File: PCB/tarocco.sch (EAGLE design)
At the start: 42 parts, among them IC1 CY8C4545PVI, Q1 NEXFET_SINGLECSD18537NQ5A, Q2 NEXFET_SINGLECSD18537NQ5A, Q3 NEXFET_SINGLECSD18537NQ5A, Q4 NEXFET_SINGLECSD18537NQ5A

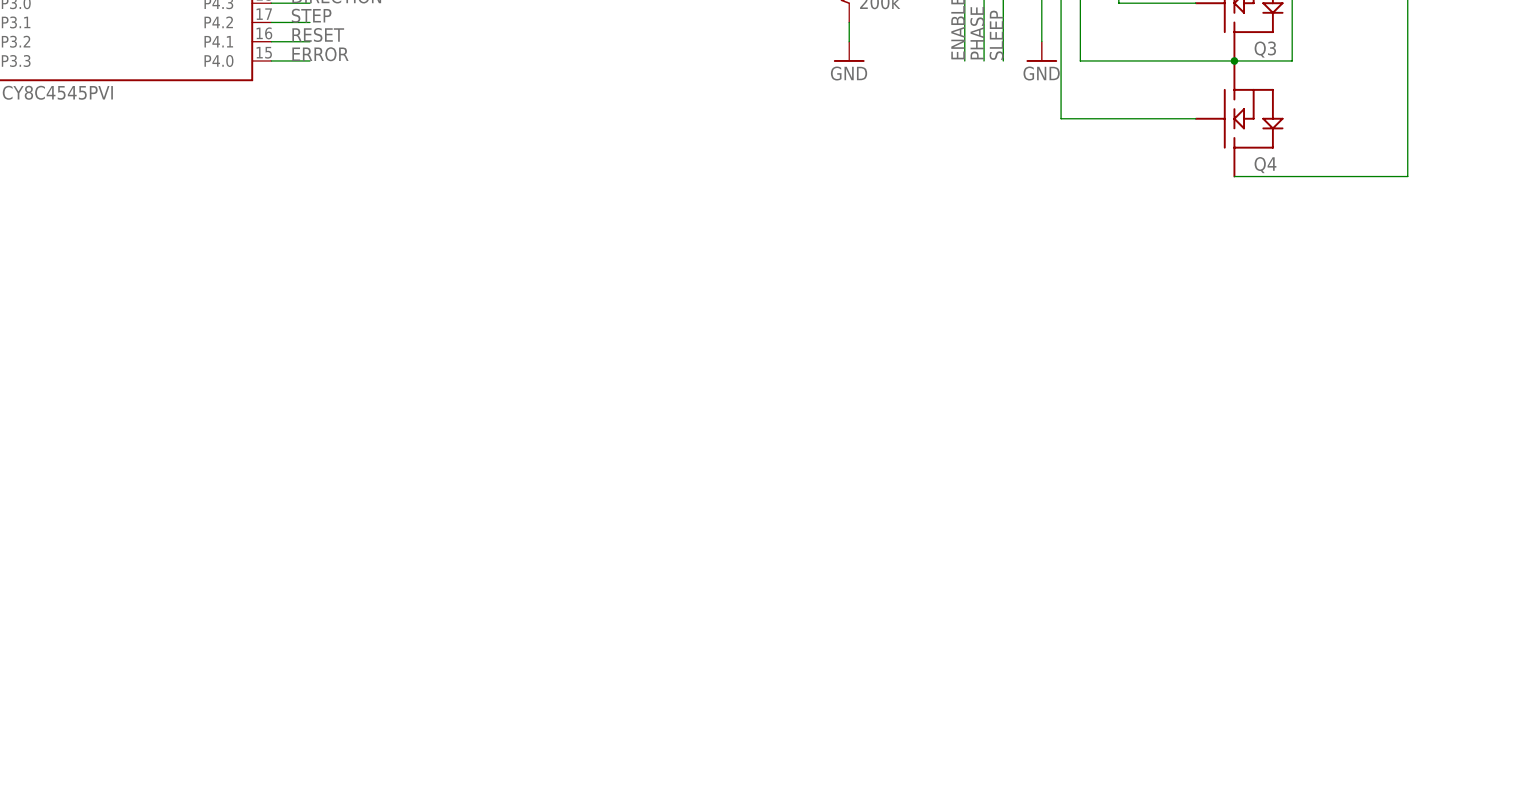
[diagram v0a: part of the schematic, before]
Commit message: Initial Commit of Schematic
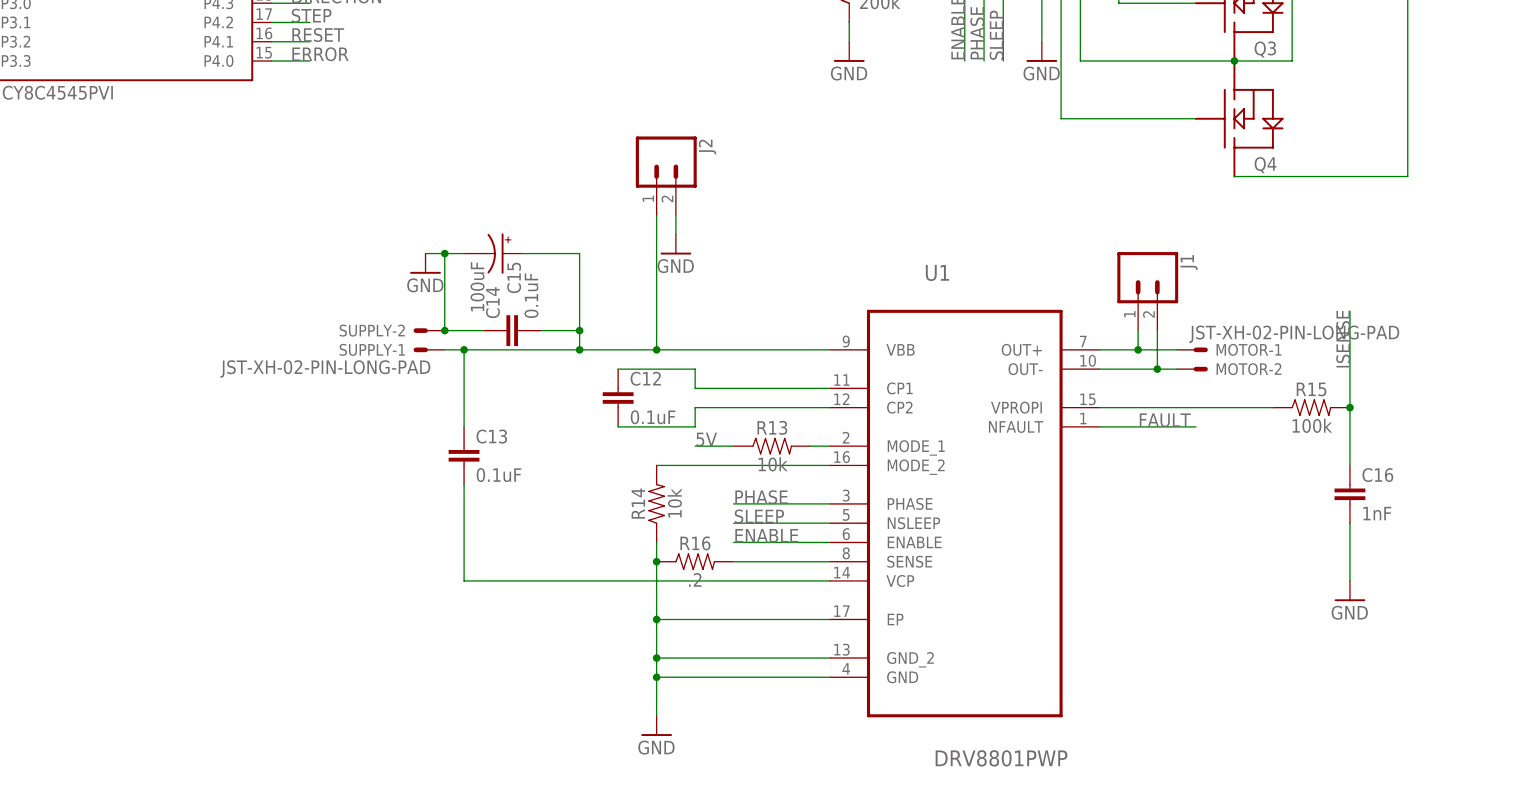
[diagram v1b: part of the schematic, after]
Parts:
- added C12: 0.1uF, SparkFun-Capacitors:0.1UF-0603-100V-10%
- added C13, C14: 0.1uF, SparkFun-Capacitors:0.1UF-0603-25V-(+80/-20%)
- added C15: 100uF, SparkFun-Capacitors:100UF-POLAR-RADIAL-2.5MM-25V-20%
- added C16: 1nF, SparkFun-Capacitors:1.0NF/1000PF-0603-50V-10%
- added J1, J2: (no value), SparkFun-Connectors:CONN_02PTH3
- added MOTOR, SUPPLY: JST-XH-02-PIN-LONG-PAD, JST XH Connectors v1-0:JST-XH-02-PIN-LONG-PAD
- added R13, R14: 10k, SparkFun-Resistors:10KOHM-0603-1/10W-1%
- added R15: 100k, SparkFun-Resistors:100KOHM-0603-1/10W-1%
- added R16: .2, SparkFun-Resistors:510OHM-2010-1/2W-5%
- added U1: DRV8801PWP, DRV8801PWP:DRV8801PWP
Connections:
- new net N$26: C13.1, C14.2, C15.+, J2.1, SUPPLY-1.S, U1.VBB
- new net N$27: R15.1, U1.VPROPI
- new net N$28: C12.1, U1.CP1
- new net N$30: C12.2, U1.CP2
- new net N$31: C13.2, U1.VCP
- new net N$32: R14.2, U1.MODE_2
- new net N$36: R16.2, U1.SENSE
- new net N$37: J1.1, MOTOR-1.S, U1.OUT+
- new net N$38: J1.2, MOTOR-2.S, U1.OUT-
- new net N$9: R13.2, U1.MODE_1
- net 5V: now also R13.1
- net ENABLE: now also U1.ENABLE
- net FAULT: now also U1.NFAULT
- net GND: now also C14.1, C15.-, C16.2, J2.2, R14.1, R16.1, SUPPLY-2.S, U1.EP, U1.GND, U1.GND_2
- net ISENSE: now also C16.1, R15.2
- net PHASE: now also U1.PHASE
- net SLEEP: now also U1.NSLEEP

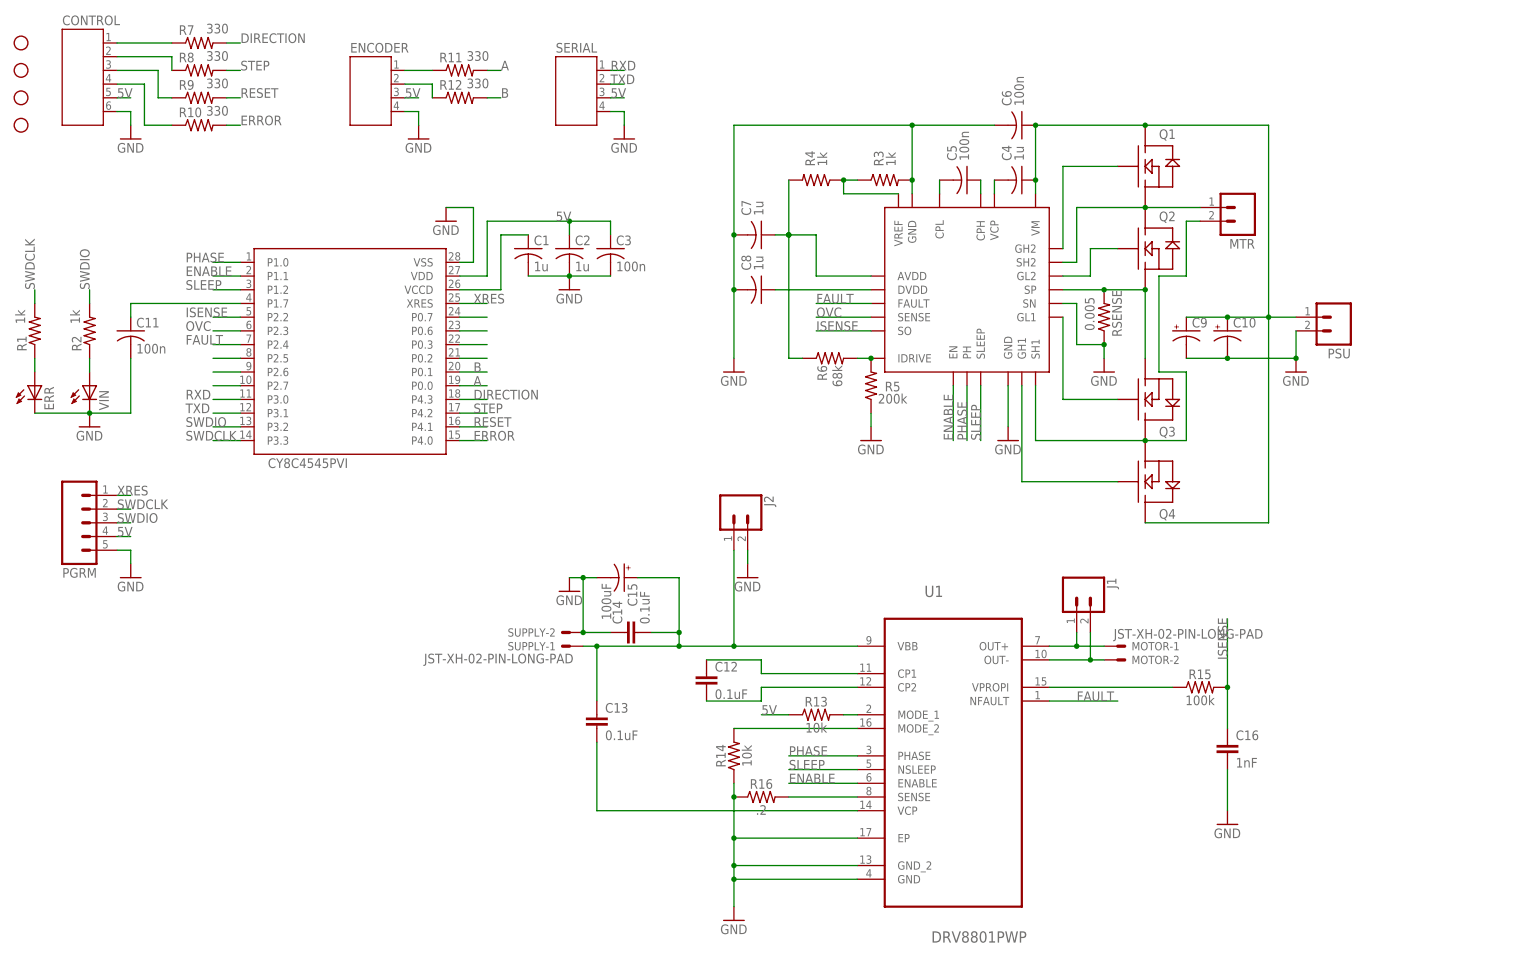
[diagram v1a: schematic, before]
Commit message: Starting BRD from scratch
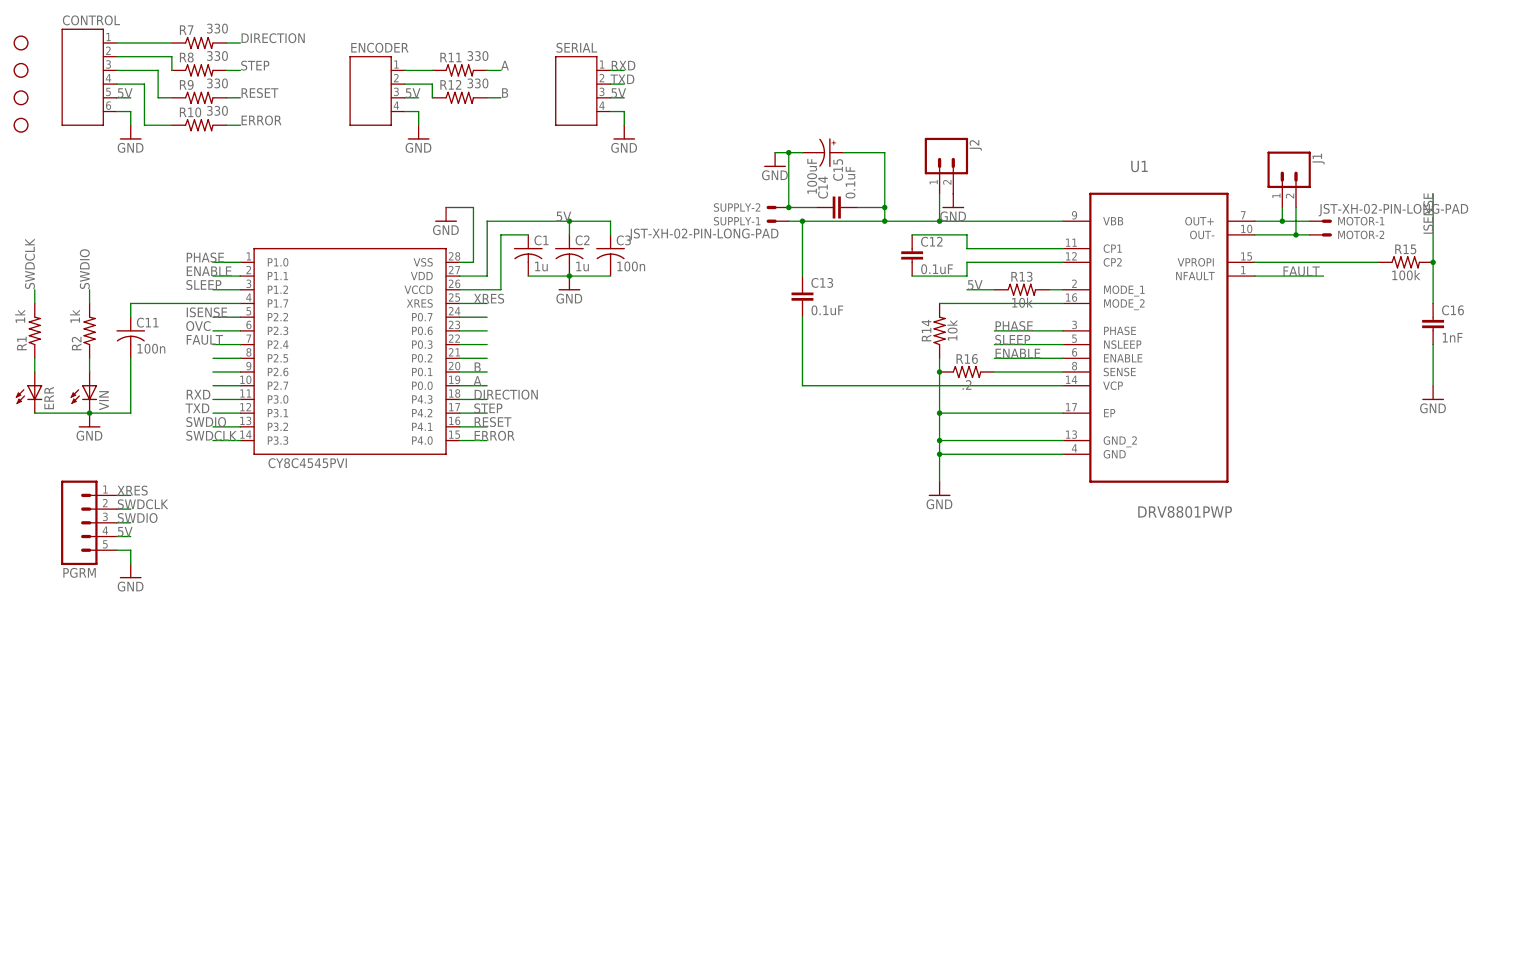
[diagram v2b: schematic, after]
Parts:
- removed 8701: DRV8701, drv8x:DRV8701
- removed C10, C9: (no value), adafruit:CPOL-USE3.5-8
- removed C4, C7, C8: 1u, adafruit:C-USC0603
- removed C5, C6: 100n, adafruit:C-USC0603
- removed MTR, PSU: M023.5MM, SparkFun-Connectors:M023.5MM
- removed Q1, Q2, Q3, Q4: NEXFET_SINGLECSD18537NQ5A, mosfet:NEXFET_SINGLECSD18537NQ5A
- removed R3, R4: 1k, adafruit:R-US_R0603
- removed R5: 200k, adafruit:R-US_R0603
- removed R6: 68k, adafruit:R-US_R0603
- removed RSENSE: 0.005, adafruit:R-US_R2512
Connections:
- removed net N$1: 8701.GL1, Q3.GATE
- removed net N$11: 8701.VCP, C4.2
- removed net N$12: 8701.CPL, C5.2
- removed net N$13: 8701.CPH, C5.1
- removed net N$15: 8701.VREF, R3.1, R4.1
- removed net N$16: 8701.AVDD, C7.1, R4.2, R6.1
- removed net N$17: 8701.DVDD, C8.1
- removed net N$2: 8701.SH1, MTR.2, Q3.DRAIN, Q4.SOURCE
- removed net N$21: 8701.IDRIVE, R5.2, R6.2
- removed net N$23: 8701.VM, C10.+, C4.1, C6.1, C9.+, PSU.1, Q1.DRAIN, Q4.DRAIN
- removed net N$3: 8701.SH2, MTR.1, Q1.SOURCE, Q2.DRAIN
- removed net N$4: 8701.GH2, Q1.GATE
- removed net N$5: 8701.SP, Q2.SOURCE, Q3.SOURCE, RSENSE.2
- removed net N$6: 8701.GL2, Q2.GATE
- removed net N$7: 8701.GH1, Q4.GATE
- net ENABLE: no longer 8701.EN
- net FAULT: no longer 8701.FAULT
- net GND: no longer 8701.GND@1, 8701.GND@2, 8701.SN, C10.-, C6.2, C7.2, C8.2, C9.-, PSU.2, R3.2, R5.1, RSENSE.1
- net ISENSE: no longer 8701.SO
- net OVC: no longer 8701.SENSE
- net PHASE: no longer 8701.PH
- net SLEEP: no longer 8701.SLEEP
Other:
- moved on the sheet: C12, C13, C14, C15, C16, J1, J2, MOTOR-1, MOTOR-2, R13, R14, R15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

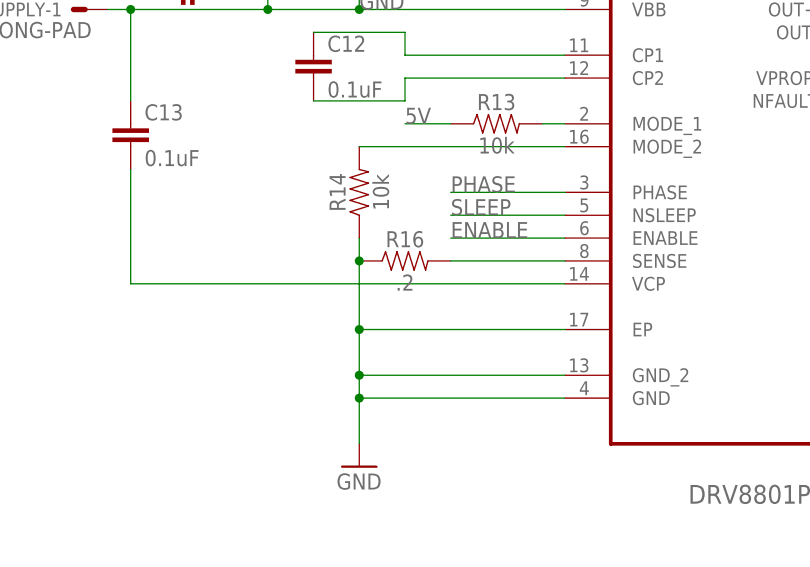
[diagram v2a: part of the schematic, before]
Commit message: Time to sleep, routing is hard
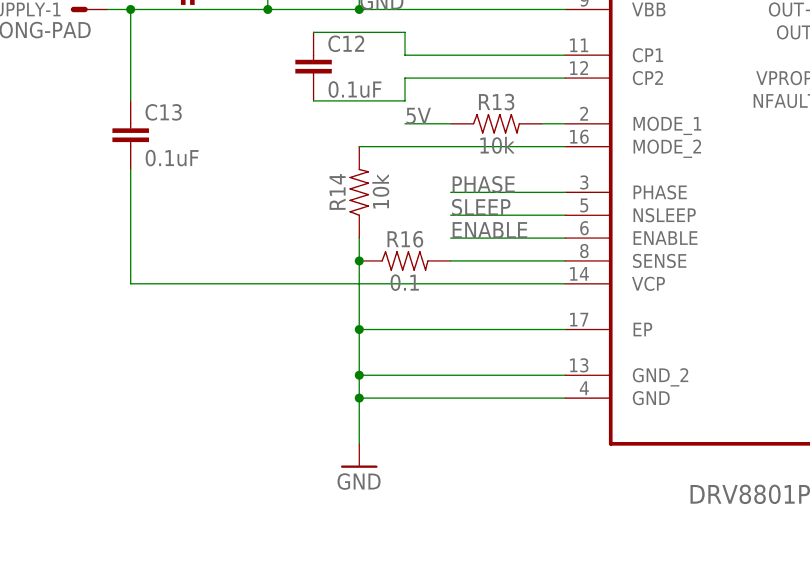
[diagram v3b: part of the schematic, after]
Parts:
- R16: value .2 -> 0.1; device SparkFun-Resistors:510OHM-2010-1/2W-5% -> SparkFun-Resistors:0.1OHM-1210-1/2W-1%
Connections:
- net N$37 renamed VMOT+
- net N$38 renamed VMOT-
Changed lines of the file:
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@@
 <part name="C16" library="SparkFun-Capacitors" deviceset="1.0NF/1000PF" device="-0603-50V-10%" value="1nF"/>
 <part name="GND15" library="SparkFun-Aesthetics" deviceset="GND" device=""/>
-<part name="R16" library="SparkFun-Resistors" deviceset="510OHM" device="-2010-1/2W-5%" value=".2"/>
+<part name="R16" library="SparkFun-Resistors" deviceset="0.1OHM" device="-1210-1/2W-1%" value="0.1"/>
 <part name="MOTOR" library="JST XH Connectors v1-0" deviceset="JST-XH-02-PIN" device="-LONG-PAD"/>
 <part name="J1" library="SparkFun-Connectors" deviceset="CONN_02" device="PTH3"/>
@@
 </segment>
 </net>
-<net name="N$37" class="0">
+<net name="VMOT+" class="0">
 <segment>
 <pinref part="MOTOR" gate="-1" pin="S"/>
@@
 </segment>
 </net>
-<net name="N$38" class="0">
+<net name="VMOT-" class="0">
 <segment>
 <pinref part="MOTOR" gate="-2" pin="S"/>
